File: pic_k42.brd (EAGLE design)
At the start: 130.5 x 111.1 mm, 65 parts, among them IC1 PIC18F57K42-E_PT, IC2 REF3440IDBVR, IC3 MAX232, IC4 ILAMP, K1 G6K-2P, Q1 ASF1, X1 RX-2, X10 J1, X11 22-23-2021, X2 TX-2, X3 RESETJMP, X4 MINI-USB-UX60A-MB-5ST, X5 PORTA, X6 PORTD, X7 PORTB, X8 J3, X9 J2

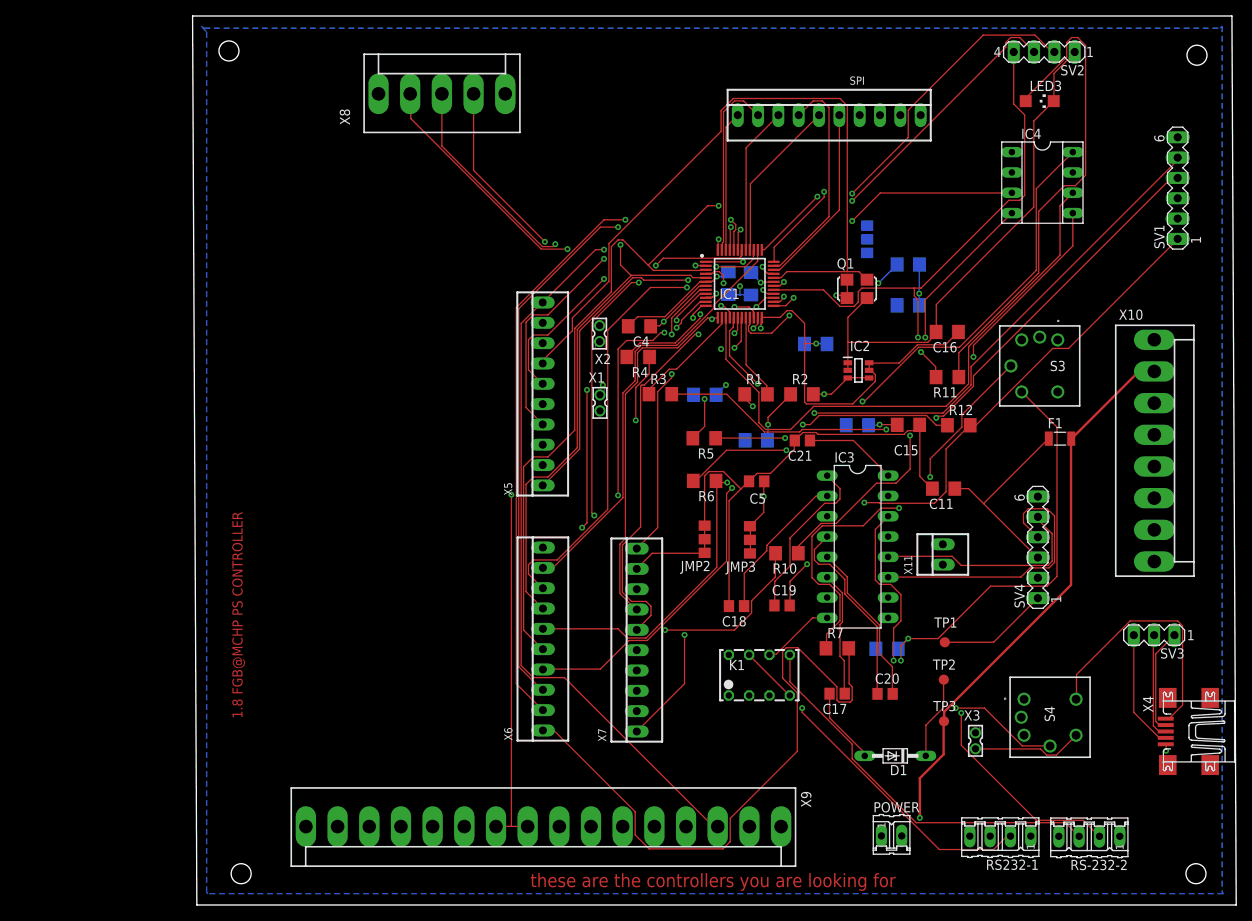
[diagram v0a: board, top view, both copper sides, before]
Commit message: up
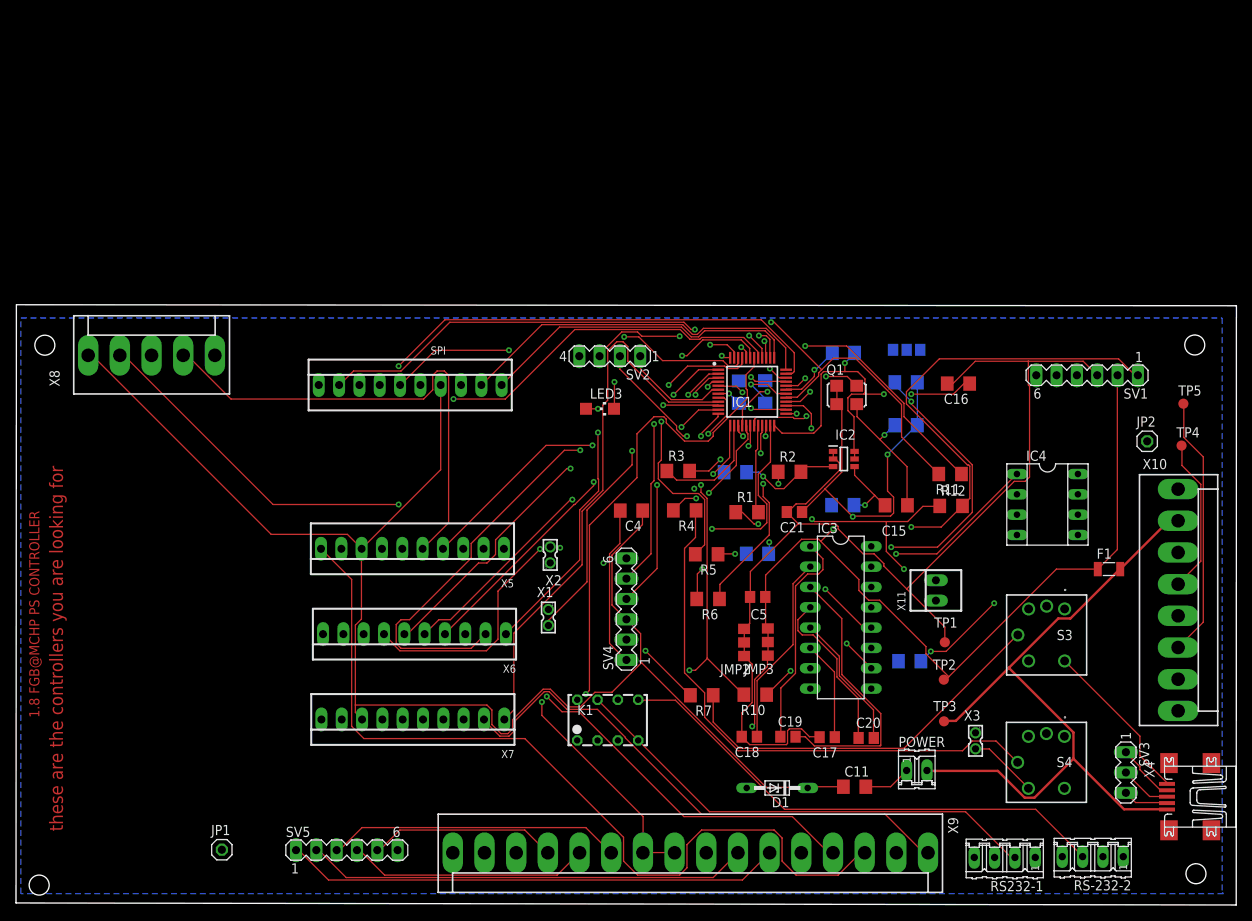
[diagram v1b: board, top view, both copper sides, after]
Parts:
- added JP1, JP2: GND, pinhead:1X01
- added SV5: ANA JUMPER, con-lstb:MA06-1
- added TP4, TP5: TPB1,27, testpad:B1,27
- moved LED3 67.1 mm to (28.8, 41.4)
- moved SV2 66.3 mm to (30.0, 48.0)
- moved SPI 62.3 mm to (5.03, 44.3)
- moved SV4 52.0 mm to (32.1, 16.3)
- moved X8 48.8 mm to (-27.3, 48.1)
- moved IC4 40.2 mm to (84.7, 29.4)
- moved C11 38.9 mm to (60.6, -5.87), turned to 0 degrees
- moved S3 33.6 mm to (84.6, 13.1)
- moved X7 29.7 mm to (5.36, 2.54), turned to 180 degrees
- moved X2 28.3 mm to (22.5, 23.1)
- moved X1 27.6 mm to (22.3, 15.3)
- moved SV1 26.0 mm to (89.6, 45.6), turned to 180 degrees
- moved X5 25.3 mm to (5.31, 23.9), turned to 180 degrees
- moved C4 23.1 mm to (32.7, 28.7)
- moved R4 20.0 mm to (39.3, 28.7)
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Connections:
- new net N$73: TP4.TP, X10.4
- new net N$74: TP5.TP, X10.6
- new net N$76: SV5.1, X9.6
- new net N$77: SV5.2, X9.7
- new net N$79: SV5.3, X9.11
- new net N$80: SV5.4, X9.12
- new net N$81: SV5.5, X9.13
- net N$54: now also X9.1
- net N$66: now also X9.2
- net RAW_VDD: now also X4.1
- net VDD: no longer X4.1
- net VSS: now also JP1.1, JP2.1, SV5.6, X9.5, X9.8
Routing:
- net VDD: track 74.3 -> 373.6 mm, vias 8 -> 6
- net N$52: track 169.7 -> 81.7 mm, vias 1 -> 3
- net N$76: track 0.00 -> 62.2 mm
- net N$54: track 65.9 -> 127.7 mm, vias 3 -> 1
- net N$77: track 0.00 -> 55.4 mm
- net N$66: track 59.0 -> 112.6 mm
- net N$39: track 127.8 -> 171.1 mm, vias 2 -> 1
- net N$29: track 17.5 -> 57.3 mm, vias 0 -> 1
- net N$31: track 18.5 -> 56.3 mm, vias 0 -> 1
- net N$79: track 0.00 -> 36.8 mm
- net N$35: track 77.3 -> 114.0 mm, vias 2 -> 1
- net N$20: track 102.8 -> 70.0 mm, vias 1 -> 2
- net N$74: track 0.00 -> 32.8 mm
- net N$32: track 28.0 -> 60.4 mm, vias 0 -> 1
- net N$30: track 23.0 -> 54.9 mm, vias 0 -> 2
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- removed copper zone on layer 15, net VDD
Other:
- board size 130.5 x 111.1 mm -> 152.6 x 75 mm
